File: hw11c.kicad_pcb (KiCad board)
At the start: 2 copper layers, 49 x 27.5 mm, 87 parts, among them Q1 KX-7_12MHZ, SW1 BUTT1, SW2 BUTT2, X1 ~RESET, X10 PIO2.8, X11 PIO1.4, X12 ADC3, X13 PIO0.8, X14 PIO0.9, X15 MAT0, X16 PIO0.6, X17 PIO0.7, X2 SWCLK, X3 SWDIO, X4 SSEL1, X5 SCK1, X6 MISO1, X7 MOSI1, X8 PIO2.6, X9 PIO2.7

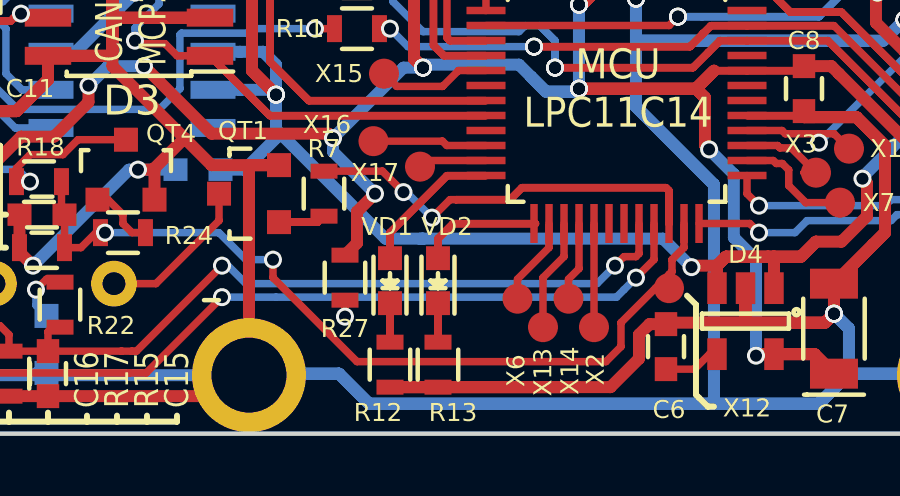
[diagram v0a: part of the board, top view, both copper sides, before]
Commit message: Add X18 pad.
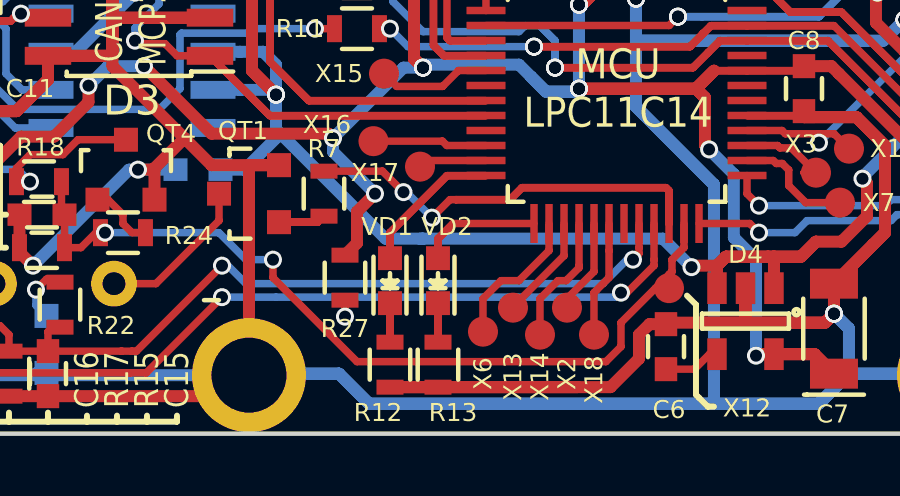
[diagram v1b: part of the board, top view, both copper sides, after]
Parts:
- added X18: ADC6, libs:PAD, F.Cu at (77.0, 74.2)
- moved X6 1.59 mm to (73.3, 74.1)
- moved X14 1.53 mm to (75.2, 74.2)
- moved X13 1.19 mm to (74.3, 73.3)
- moved X2 1.11 mm to (76.1, 73.3)
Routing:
- net Net-(D1-Pad30): track 0.00 -> 3.71 mm
- net Net-(D1-Pad25): track 8.32 -> 5.42 mm
- net /SO: track 2.94 -> 4.87 mm
- net Net-(D1-Pad28): track 2.65 -> 4.40 mm
